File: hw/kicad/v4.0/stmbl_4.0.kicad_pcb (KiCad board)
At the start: 2 copper layers, 100 x 100 mm, 433 parts, among them J1 RJ45_LED, J2 RJ45_LED, J3 RJ45_LED, P1 USB_OTG, P10 CONN_02X06, P11 USB_OTG, P12 CONN_01X04, P13 CONN_01X04, P14 CONN_01X04, P15 CONN_01X02, P2 CONN_01X02, P3 CONN_01X02, P4 CONN_01X02, P5 CONN_01X06, P6 CONN_01X02, P7 CONN_01X04, P8 CONN_01X03, P9 CONN_01X06, Q1 IRLML6344, Q2 IRLML6344, Q3 IRLML6344, Q4 IRLML6344, Q5 IRLML6344, T1 testpoint, T2 testpoint, T44 testpoint, T45 testpoint, T46 testpoint, U1 USBLC6-4SC6, U10 SN65176B, U11 SN65176B, U12 IRAM256a, U13 ACT4088, U14 SN65176B, U15 SN65176B, U16 SN65176B, U17 SN65176B, U18 SN65176B, U19 SN65176B, U2 zldo1117, U20 USBLC6-4SC6, U21 USBLC6-4SC6, U22 USBLC6-4SC6, U23 USBLC6-4SC6, U24 non_plated, U25 STM32F303CBTx, U26 STM32F405VG, U27 ACT4088, U28 ACT4088, U29 USBLC6-4SC6, U3 SI8621, U30 non_plated, U31 non_plated, U32 non_plated, U33 heatsink, U34 fan, U35 non_plated, U36 non_plated, U37 non_plated, U39 non_plated, U4 ACT4088, U5 LNK304D, U6 LM358, U7 LM358, U8 SN65176B, U9 SN65176B, Y1 8M, Y2 8M

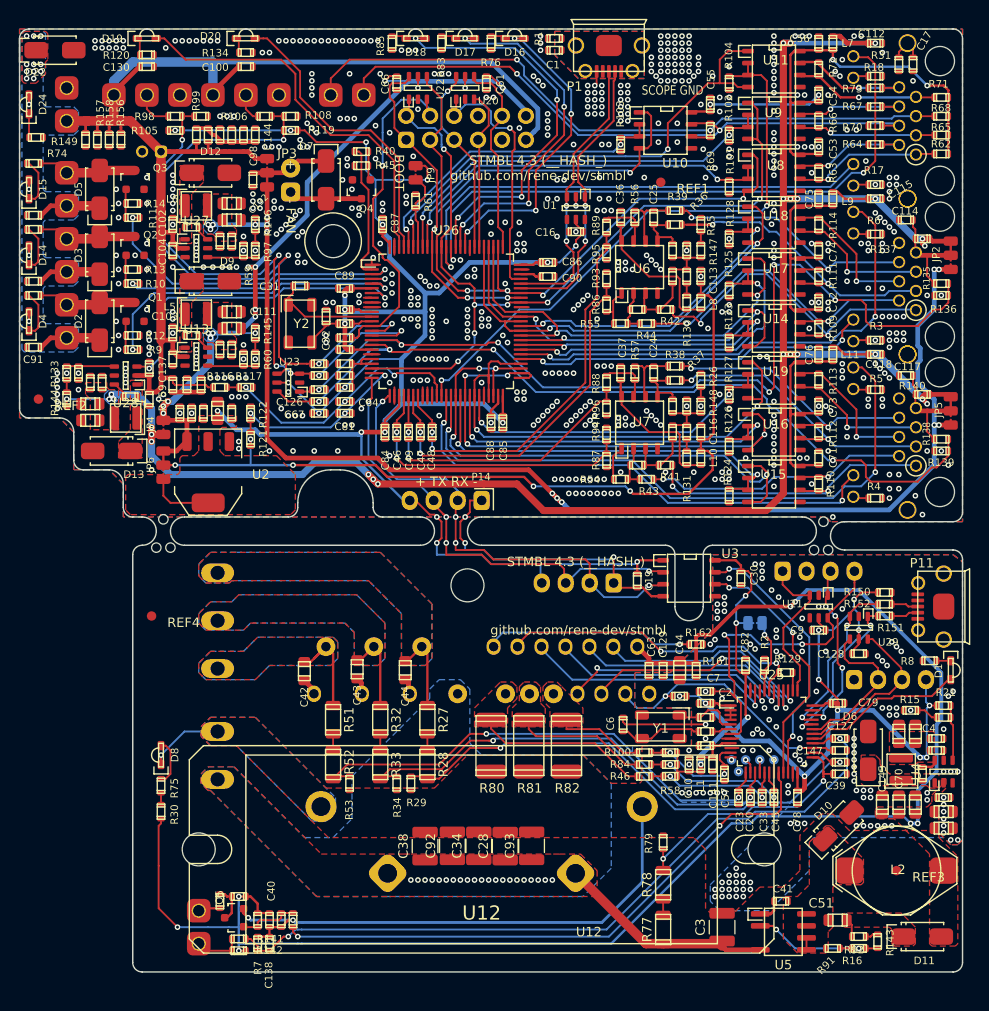
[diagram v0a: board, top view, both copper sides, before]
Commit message: couple other PCB changes
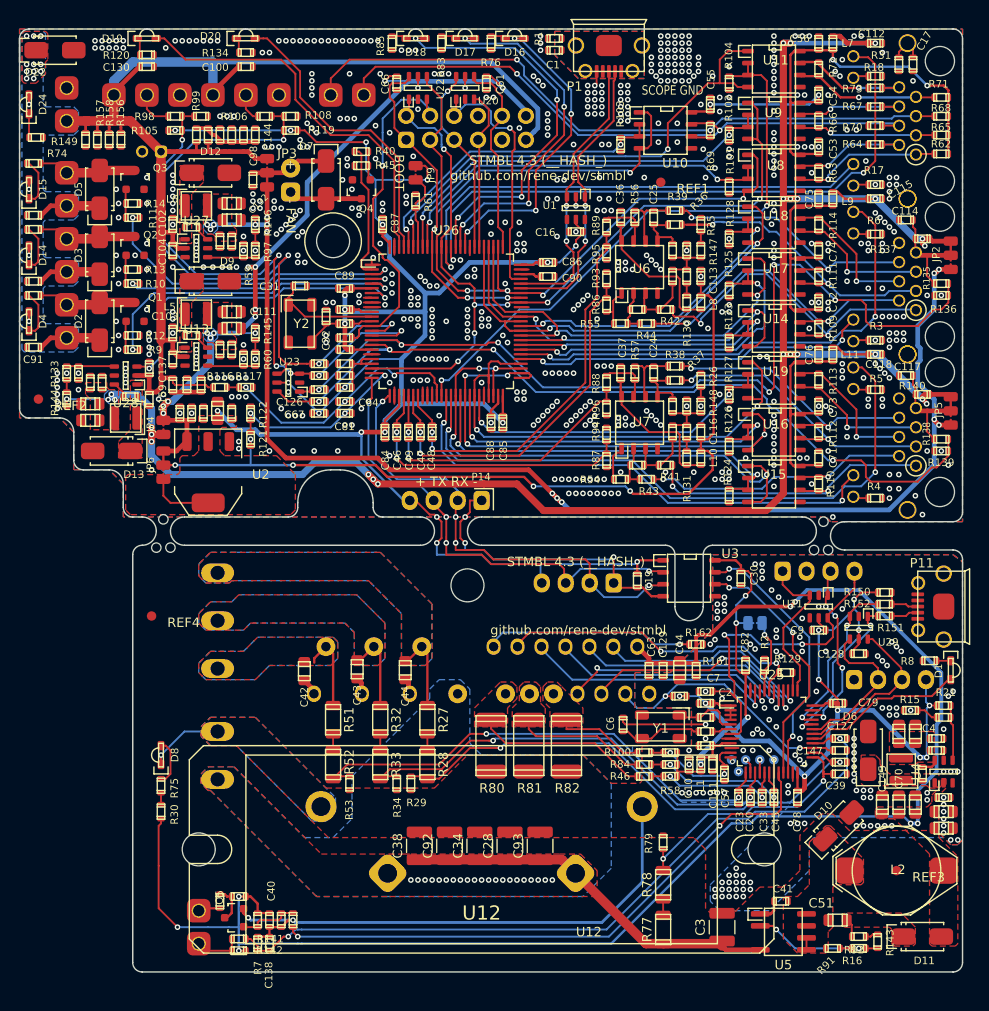
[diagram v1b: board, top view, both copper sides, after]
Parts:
- moved C93 0.90 mm to (153.2, 136.4)
- moved C38 0.60 mm to (140.4, 136.4)
- moved C28 0.50 mm to (150.0, 136.4)
- moved C92 0.30 mm to (143.6, 136.4)
- moved C34 0.10 mm to (146.8, 136.4)
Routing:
- net VPP: track 22.9 -> 40.1 mm
- net /hv/back-emf/W: track 11.2 -> 8.68 mm
- net +12V: track 140.7 -> 141.8 mm
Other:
- net class Default: via_dia 0.6 -> 0.5
- net class UVW: via_dia 0.6 -> 0.5
- net class UVW_L: via_dia 0.6 -> 0.5
- net class VPP: via_dia 0.6 -> 0.5
- rule via_min_size: 0.6 -> 0.5
